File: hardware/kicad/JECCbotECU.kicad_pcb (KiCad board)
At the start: 2 copper layers, 100 x 60 mm, 74 parts, among them CN1 ADAFRUIT_FEATHER, P1 USB_B, U1 STM32F103C8Tx, U2 BSS138, U3 BSS138, U4 BNO055, U5 TPS54335A, U6 GAPTEC_6S8W4_1.6RP, U7 LT1117, Y1 Crystal_Small

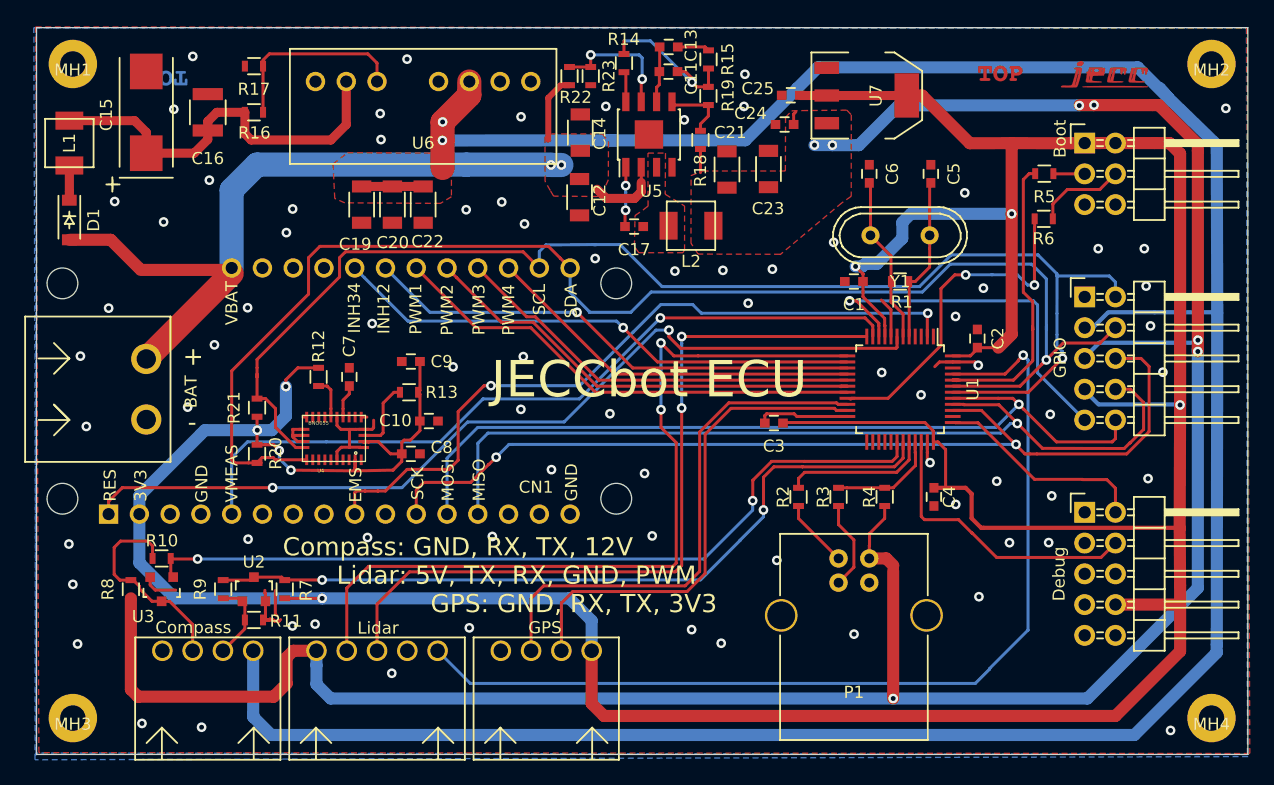
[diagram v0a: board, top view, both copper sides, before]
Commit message: improved layout
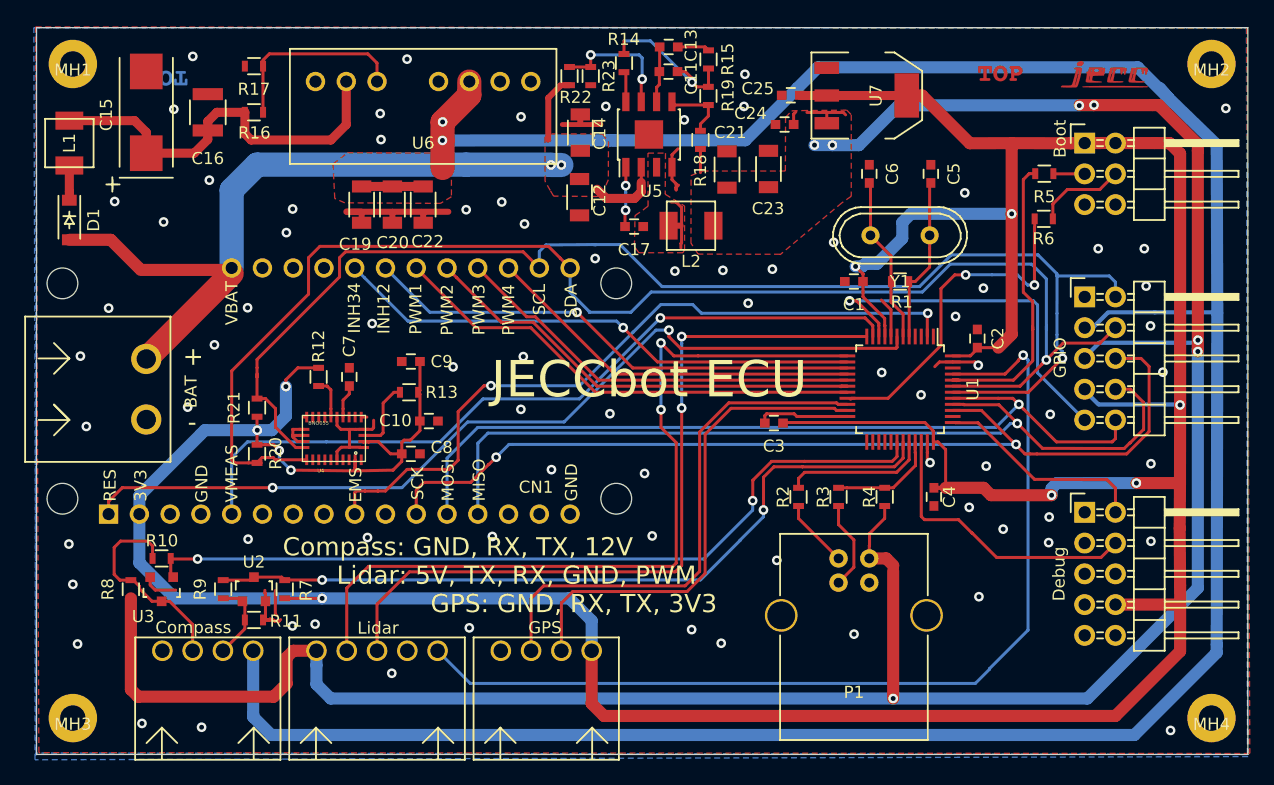
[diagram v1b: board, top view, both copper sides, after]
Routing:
- net GND: track 53.4 -> 72.9 mm, vias 77 -> 78
- net /power/REG_5V_PH: track 0.00 -> 5.44 mm
- net +5V: track 210.9 -> 215.1 mm
- net +3V3: track 330.3 -> 328.8 mm, vias 8 -> 10
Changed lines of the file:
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@@
     (thickness 1.6)
     (drawings 29)
-    (tracks 898)
+    (tracks 937)
     (zones 0)
     (modules 74)
@@
   (gr_line (start 190 40) (end 190 100) (layer Edge.Cuts) (width 0.05))
   (gr_line (start 90 40) (end 190 40) (layer Edge.Cuts) (width 0.05))
+  (segment (start 156.6 47) (end 156.8 47.2) (width 0.25) (layer F.Cu) (net 12))
+  (segment (start 143.2 58.2) (end 143.2 57.813062) (width 0.25) (layer F.Cu) (net 11))
+  (segment (start 143.253161 57.759901) (end 143.253161 54.853161) (width 0.25) (layer F.Cu) (net 11))
+  (segment (start 143.2 57.813062) (end 143.253161 57.759901) (width 0.25) (layer F.Cu) (net 11))
+  (segment (start 143.253161 54.853161) (end 142.8 54.4) (width 0.25) (layer F.Cu) (net 11))
+  (segment (start 142.8 54.4) (end 142.4 54.4) (width 0.25) (layer F.Cu) (net 11))
   (segment (start 109.714999 86.599999) (end 109.714999 88.419639) (width 0.25) (layer F.Cu) (net 1))
   (segment (start 109.71784 86.46668) (end 109.71784 86.597158) (width 0.25) (layer F.Cu) (net 1))
   (segment (start 109.71784 86.597158) (end 109.714999 86.599999) (width 0.25) (layer F.Cu) (net 1))
   (segment (start 109.714999 88.419639) (end 109.83976 88.5444) (width 0.25) (layer F.Cu) (net 1))
-  (via (at 165.8874 79.35976) (size 0.8) (drill 0.4) (layers F.Cu B.Cu) (net 1))
+  (via (at 167 79.6) (size 0.8) (drill 0.4) (layers F.Cu B.Cu) (net 1))
   (via (at 166.63416 53.63972) (size 0.8) (drill 0.4) (layers F.Cu B.Cu) (net 1))
   (segment (start 156.94 72.1) (end 152.76532 72.1) (width 0.25) (layer F.Cu) (net 1))
@@
   (segment (start 150.26808 71.87692) (end 150.126 72.019) (width 0.25) (layer F.Cu) (net 1))
   (segment (start 152.54224 71.87692) (end 150.26808 71.87692) (width 0.25) (layer F.Cu) (net 1))
-  (via (at 181.7624 77.22616) (size 0.8) (drill 0.4) (layers F.Cu B.Cu) (net 1))
+  (via (at 182 76) (size 0.8) (drill 0.4) (layers F.Cu B.Cu) (net 1))
   (segment (start 114.804 74.989) (end 115.15256 74.64044) (width 0.25) (layer F.Cu) (net 1))
   (segment (start 114.804 75.6765) (end 114.804 74.989) (width 0.25) (layer F.Cu) (net 1))
@@
   (via (at 136.1186 59.06008) (size 0.8) (drill 0.4) (layers F.Cu B.Cu) (net 1))
   (via (at 159.77616 68.46824) (size 0.8) (drill 0.4) (layers F.Cu B.Cu) (net 1))
-  (via (at 169.27068 77.4446) (size 0.8) (drill 0.4) (layers F.Cu B.Cu) (net 1))
-  (via (at 173.8122 78.65364) (size 0.8) (drill 0.4) (layers F.Cu B.Cu) (net 1))
+  (via (at 168.4 76.2) (size 0.8) (drill 0.4) (layers F.Cu B.Cu) (net 1))
+  (via (at 173.6 80.4) (size 0.8) (drill 0.4) (layers F.Cu B.Cu) (net 1))
   (via (at 173.5582 82.51444) (size 0.8) (drill 0.4) (layers F.Cu B.Cu) (net 1))
-  (via (at 170.32224 82.51952) (size 0.8) (drill 0.4) (layers F.Cu B.Cu) (net 1))
+  (via (at 169.8 81.4) (size 0.8) (drill 0.4) (layers F.Cu B.Cu) (net 1))
   (via (at 173.69028 71.92264) (size 0.8) (drill 0.4) (layers F.Cu B.Cu) (net 1))
   (via (at 163.02228 70.31736) (size 0.8) (drill 0.4) (layers F.Cu B.Cu) (net 1))
@@
   (via (at 168.16832 61.50864) (size 0.8) (drill 0.4) (layers F.Cu B.Cu) (net 1))
   (via (at 137 46.5) (size 0.8) (drill 0.4) (layers F.Cu B.Cu) (net 1))
+  (via (at 182 82.4) (size 0.8) (drill 0.4) (layers F.Cu B.Cu) (net 1))
+  (segment (start 142.46098 52.54888) (end 142.8 52.8879) (width 0.25) (layer F.Cu) (net 1))
+  (segment (start 142.46098 51.52388) (end 142.46098 52.54888) (width 0.25) (layer F.Cu) (net 1))
+  (segment (start 142.8 52.8879) (end 142.8 53.4) (width 0.25) (layer F.Cu) (net 1))
+  (segment (start 142.8 53.4) (end 142.8 53.2) (width 0.25) (layer F.Cu) (net 1))
+  (segment (start 142.8 53.2) (end 143 53) (width 0.25) (layer F.Cu) (net 1))
+  (segment (start 142.46098 50.49888) (end 142.95986 50) (width 0.25) (layer F.Cu) (net 1))
+  (segment (start 142.46098 51.52388) (end 142.46098 50.49888) (width 0.25) (layer F.Cu) (net 1))
+  (segment (start 134.80564 48) (end 134.89178 47.91386) (width 0.25) (layer F.Cu) (net 1))
+  (segment (start 134.89178 47.91386) (end 134.89178 47.16386) (width 0.5) (layer F.Cu) (net 1))
+  (segment (start 134.8 48) (end 134.80564 48) (width 0.25) (layer F.Cu) (net 1))
+  (segment (start 134.8 48) (end 136.6 48) (width 0.4) (layer F.Cu) (net 1))
+  (segment (start 133.4 48) (end 134.8 48) (width 0.4) (layer F.Cu) (net 1))
+  (segment (start 116.84 55.24) (end 116.8 55.2) (width 0.25) (layer F.Cu) (net 1))
+  (segment (start 116.84 56.11) (end 116.84 55.24) (width 0.5) (layer F.Cu) (net 1))
+  (segment (start 115.6 55.2) (end 116.8 55.2) (width 0.55) (layer F.Cu) (net 1))
+  (segment (start 119.38 56.11) (end 119.38 55.22) (width 0.5) (layer F.Cu) (net 1))
+  (segment (start 119.38 55.22) (end 119.4 55.2) (width 0.25) (layer F.Cu) (net 1))
+  (segment (start 116.8 55.2) (end 119.4 55.2) (width 0.5) (layer F.Cu) (net 1))
+  (segment (start 121.92 55.32) (end 121.8 55.2) (width 0.25) (layer F.Cu) (net 1))
+  (segment (start 119.4 55.2) (end 121.8 55.2) (width 0.5) (layer F.Cu) (net 1))
+  (segment (start 121.92 56.11) (end 121.92 55.32) (width 0.5) (layer F.Cu) (net 1))
+  (segment (start 121.8 55.2) (end 124 55.2) (width 0.5) (layer F.Cu) (net 1))
   (segment (start 167.088 67.1) (end 165.64 67.1) (width 0.25) (layer F.Cu) (net 2))
   (segment (start 167.628 66.56) (end 167.088 67.1) (width 0.25) (layer F.Cu) (net 2))
@@
   (segment (start 184.40908 50.39868) (end 184.40908 71.05396) (width 1) (layer F.Cu) (net 2))
   (segment (start 158.23 60.96) (end 158.23 60.335) (width 0.25) (layer F.Cu) (net 2))
-  (segment (start 184.40908 71.05396) (end 184.37352 81.32064) (width 1) (layer F.Cu) (net 2))
-  (segment (start 167.19804 78.4846) (end 167.19804 80.50784) (width 0.35) (layer F.Cu) (net 2))
-  (segment (start 166.70344 77.99) (end 167.19804 78.4846) (width 0.35) (layer F.Cu) (net 2))
   (segment (start 163.34 72.6) (end 156.94 72.6) (width 0.25) (layer F.Cu) (net 2))
   (segment (start 164.04 74.2) (end 164.04 73.3) (width 0.25) (layer F.Cu) (net 2))
@@
   (segment (start 110.03788 75.56788) (end 111.0002 76.5302) (width 0.25) (layer B.Cu) (net 2))
   (segment (start 184.332761 81.361399) (end 184.37352 81.32064) (width 0.25) (layer F.Cu) (net 2))
-  (segment (start 168.17594 81.29016) (end 184.33542 81.29016) (width 0.35) (layer F.Cu) (net 2))
   (segment (start 155.23972 45.60316) (end 161.84372 45.60316) (width 0.75) (layer F.Cu) (net 2))
   (segment (start 153.03824 45.60316) (end 153.01792 45.58284) (width 0.25) (layer F.Cu) (net 2))
@@
   (segment (start 164.04 74.2) (end 164.415 74.2) (width 0.25) (layer F.Cu) (net 2))
   (segment (start 164.084 77.99) (end 165.0492 77.98816) (width 0.35) (layer F.Cu) (net 2))
-  (segment (start 165.0492 77.98816) (end 166.70344 77.99) (width 0.35) (layer F.Cu) (net 2))
   (segment (start 158.23 60.335) (end 158.23 60.32824) (width 0.25) (layer F.Cu) (net 2))
   (via (at 157.61716 59.7154) (size 0.8) (drill 0.4) (layers F.Cu B.Cu) (net 2))
@@
   (segment (start 158.182845 59.7154) (end 158.396205 59.50204) (width 1) (layer B.Cu) (net 2))
   (segment (start 157.61716 59.7154) (end 158.182845 59.7154) (width 1) (layer B.Cu) (net 2))
-  (segment (start 167.98036 81.29016) (end 167.19804 80.50784) (width 0.35) (layer F.Cu) (net 2))
-  (segment (start 168.17594 81.29016) (end 167.98036 81.29016) (width 0.35) (layer F.Cu) (net 2))
+  (segment (start 165.0492 77.98816) (end 168.18816 77.98816) (width 1) (layer F.Cu) (net 2))
+  (via (at 173.8 78.6) (size 0.8) (drill 0.4) (layers F.Cu B.Cu) (net 2))
+  (segment (start 168.18816 77.98816) (end 168.8 78.6) (width 1) (layer F.Cu) (net 2))
+  (segment (start 168.8 78.6) (end 173.8 78.6) (width 1) (layer F.Cu) (net 2))
+  (segment (start 173.8 78.034315) (end 174.234315 77.6) (width 1) (layer B.Cu) (net 2))
+  (segment (start 173.8 78.6) (end 173.8 78.034315) (width 1) (layer B.Cu) (net 2))
+  (segment (start 174.234315 77.6) (end 180.8 77.6) (width 1) (layer B.Cu) (net 2))
+  (via (at 180.8 77.6) (size 0.8) (drill 0.4) (layers F.Cu B.Cu) (net 2))
+  (segment (start 180.8 77.6) (end 184.4 77.6) (width 1) (layer F.Cu) (net 2))
+  (segment (start 184.40908 71.05396) (end 184.4 77.6) (width 1) (layer F.Cu) (net 2))
+  (segment (start 184.4 77.6) (end 184.37352 81.32064) (width 1) (layer F.Cu) (net 2))
   (segment (start 162.04 65.5) (end 162.04 60.96) (width 0.25) (layer F.Cu) (net 3))
   (segment (start 163.73094 58.211466) (end 163.73094 57.15) (width 0.25) (layer F.Cu) (net 3))
@@
   (segment (start 138.58424 55.12378) (end 138.63066 55.07736) (width 0.25) (layer F.Cu) (net 10))
   (segment (start 138.58424 56.42102) (end 138.58424 55.12378) (width 0.25) (layer F.Cu) (net 10))
+  (segment (start 143.17816 56.3499) (end 143.2 56.32806) (width 0.25) (layer F.Cu) (net 11))
+  (segment (start 142.17816 56.3499) (end 143.17816 56.3499) (width 0.5) (layer F.Cu) (net 11))
   (via (at 154.22372 49.69764) (size 0.8) (drill 0.4) (layers F.Cu B.Cu) (net 12))
   (segment (start 154.2796 49.72812) (end 154.2542 49.72812) (width 0.25) (layer F.Cu) (net 12))
@@
   (segment (start 182.64564 46.39564) (end 182.11292 46.39564) (width 1) (layer F.Cu) (net 12))
   (segment (start 185.87212 49.62212) (end 182.64564 46.39564) (width 1) (layer F.Cu) (net 12))
+  (segment (start 155.23972 47.03972) (end 155.2 47) (width 0.25) (layer F.Cu) (net 12))
+  (segment (start 155.23972 47.88916) (end 155.23972 47.03972) (width 0.25) (layer F.Cu) (net 12))
+  (segment (start 153.6 47) (end 155.2 47) (width 0.25) (layer F.Cu) (net 12))
+  (segment (start 155.2 47) (end 156.6 47) (width 0.25) (layer F.Cu) (net 12))
   (via (at 142.20952 64.96812) (size 0.8) (drill 0.4) (layers F.Cu B.Cu) (net 13))
   (segment (start 142.20952 65.517882) (end 142.20952 64.96812) (width 0.25) (layer F.Cu) (net 13))
